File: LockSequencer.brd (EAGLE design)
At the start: 100 x 80 mm, 76 parts, among them IC1 4017D, IC2 NE555, K1 G2RATE-OJ, K2 G2RATE-OJ

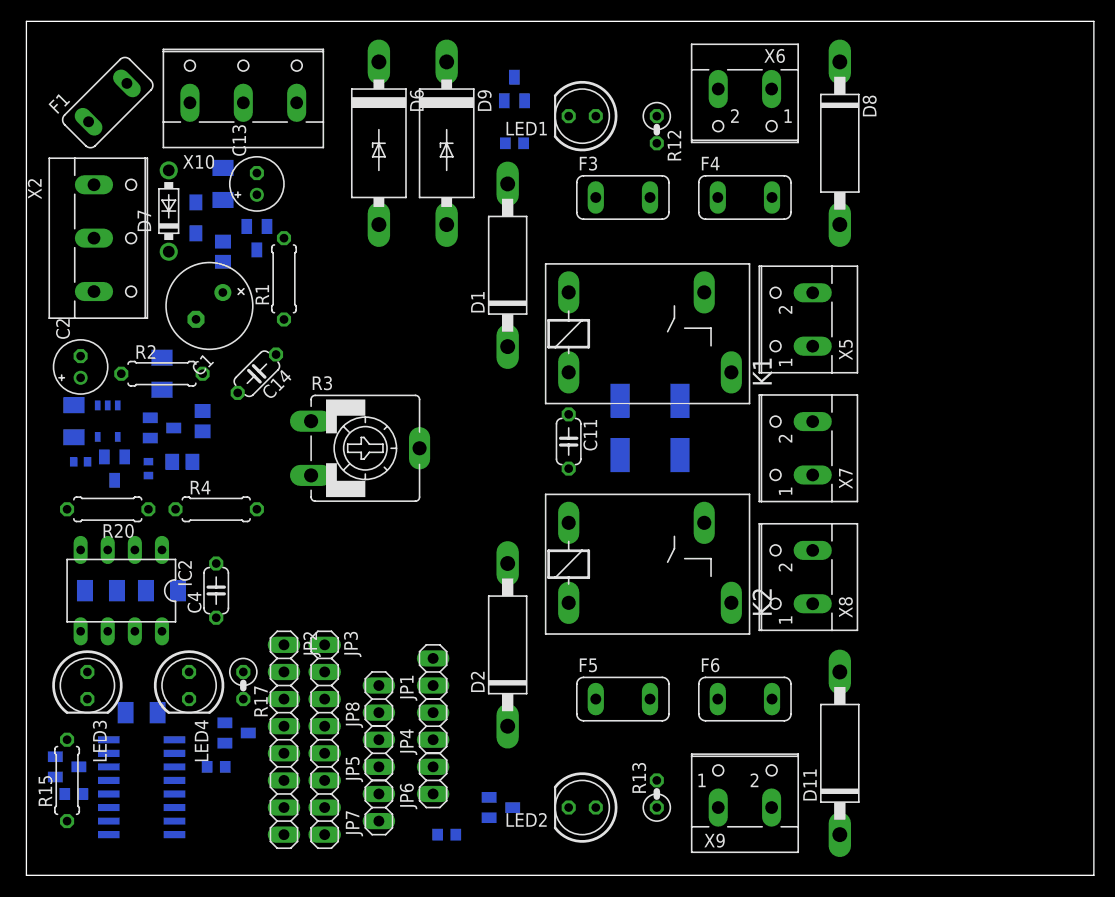
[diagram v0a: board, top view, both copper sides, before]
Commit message: Tweaked positions
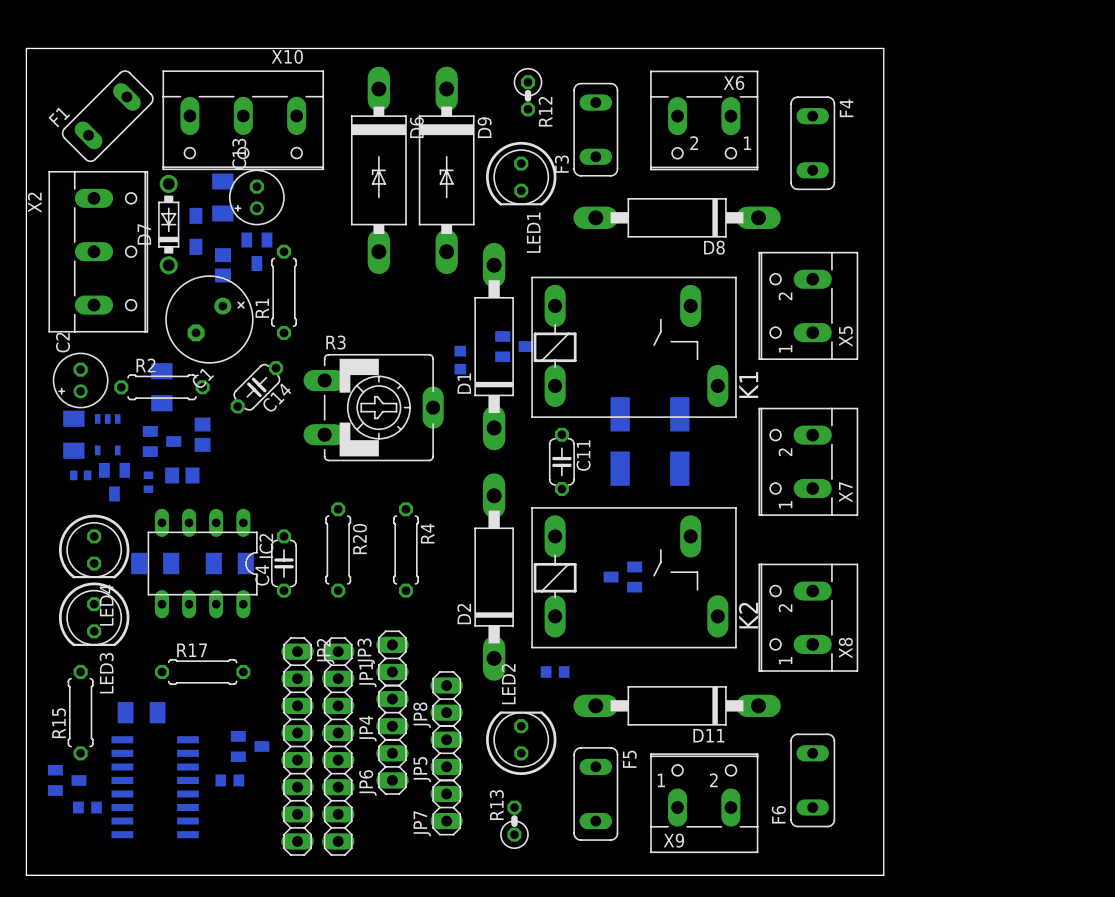
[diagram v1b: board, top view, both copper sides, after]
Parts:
- R17: device rcl:0207/2V -> rcl:0207/7
- moved T3 24.4 mm to (55.9, 27.9), turned to 270 degrees
- moved T4 24.1 mm to (45.7, 49.5), turned to 90 degrees
- moved R20 21.9 mm to (29.2, 30.5), turned to 270 degrees
- moved R10 20.9 mm to (40.6, 48.3), turned to 90 degrees
- moved R11 18.3 mm to (49.5, 19.1)
- moved R4 18.2 mm to (35.6, 30.5), turned to 270 degrees
- moved D8 16.8 mm to (61.0, 61.6), turned to 180 degrees
- moved D11 15.9 mm to (61.0, 15.9), turned to 180 degrees
- moved LED4 15.5 mm to (6.35, 30.5)
- moved R13 13.6 mm to (45.7, 5.08)
- moved R12 12.5 mm to (47.0, 73.0)
- moved F6 9.92 mm to (73.7, 8.89), turned to 90 degrees
- moved F5 9.25 mm to (53.3, 7.62), turned to 270 degrees
- moved LED2 8.54 mm to (46.4, 12.7), turned to 90 degrees
- moved F4 8.13 mm to (73.7, 68.6), turned to 270 degrees
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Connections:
- net N$21: now also X5.1; no longer X5.2
- net N$30: now also X5.2; no longer X5.1
- net N$43: now also X8.2; no longer X8.1
- net N$44: now also X8.1; no longer X8.2
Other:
- board size 100 x 80 mm -> 80.3 x 77.5 mm
